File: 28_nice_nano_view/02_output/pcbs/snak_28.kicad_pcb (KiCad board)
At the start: 2 copper layers, 114.8 x 99.6 mm, 156 parts

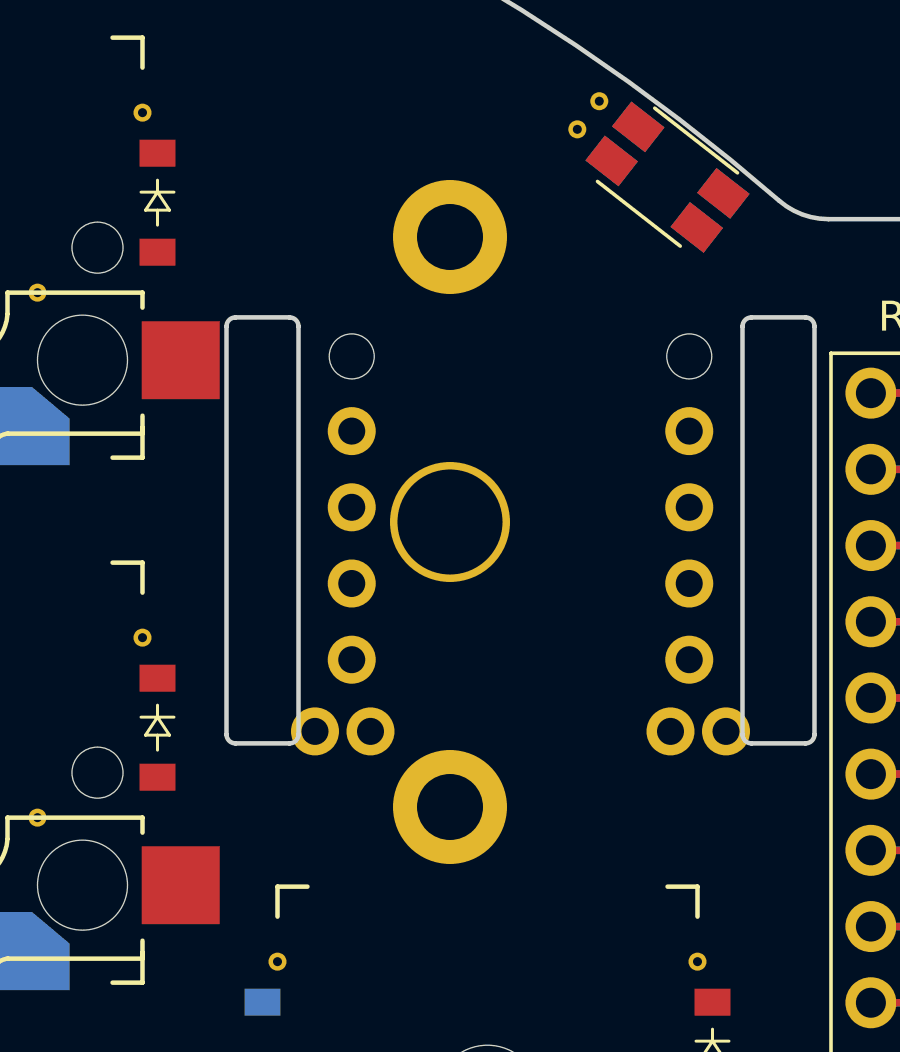
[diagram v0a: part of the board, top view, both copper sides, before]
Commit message: update
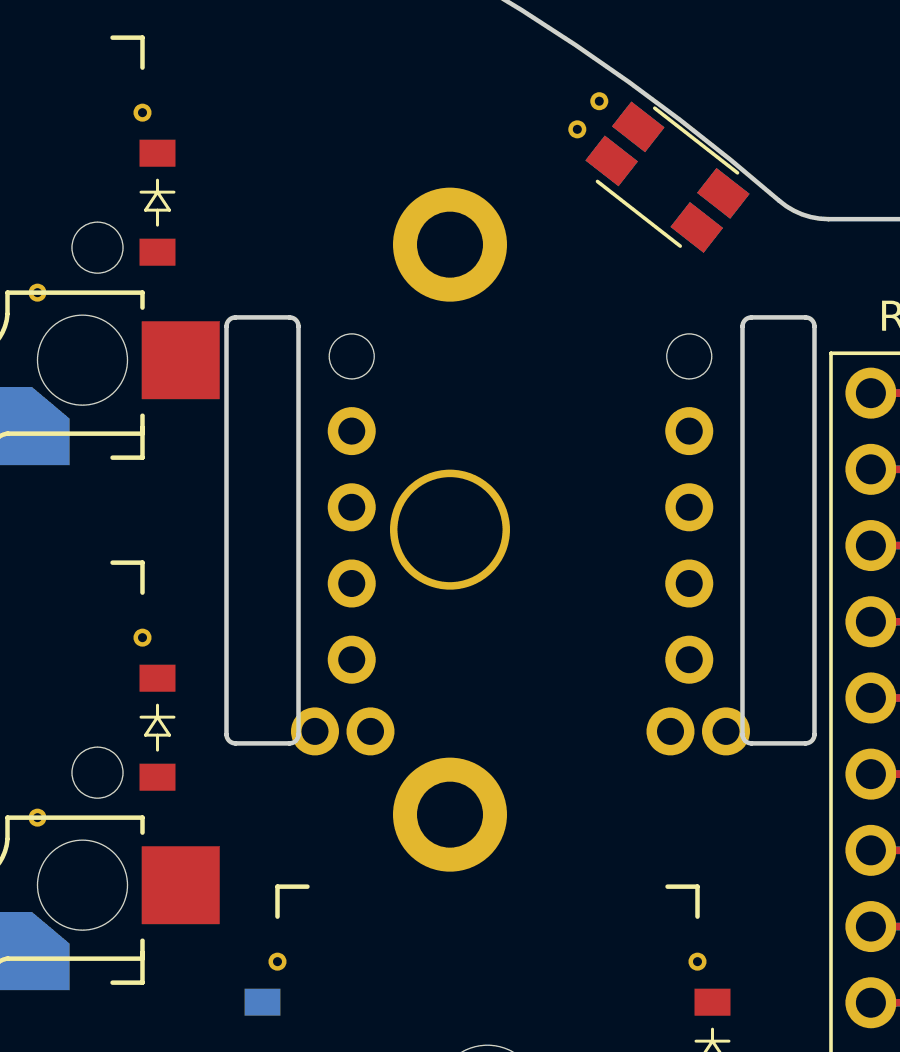
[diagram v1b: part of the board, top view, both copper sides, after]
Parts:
- moved TP1 0.26 mm to (172.8, 62.1)
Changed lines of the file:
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@@
             )
       (module trackpoint_mount_t430 (layer F.Cu)
-        (at 172.75 61.845 0)
+        (at 172.75 62.1 0)
         (attr virtual)
         (fp_text reference "TP1" (at 0 0) (layer B.SilkS) hide
@@
 (gr_circle (center 170.43886559999999 124.35568) (end 171.43886559999999 124.35568) (layer Eco1.User) (width 0.15))
 (gr_circle (center 201.925 53.975) (end 202.925 53.975) (layer Eco1.User) (width 0.15))
-(gr_circle (center 172.75 52.345) (end 173.75 52.345) (layer Eco1.User) (width 0.15))
-(gr_circle (center 172.75 71.345) (end 173.75 71.345) (layer Eco1.User) (width 0.15))
+(gr_circle (center 172.75 52.6) (end 173.75 52.6) (layer Eco1.User) (width 0.15))
+(gr_circle (center 172.75 71.6) (end 173.75 71.6) (layer Eco1.User) (width 0.15))
 (gr_line (start 93.05 89.45) (end 106.95 89.45) (angle 90) (layer Eco1.User) (width 0.15))
 (gr_line (start 106.95 89.45) (end 106.95 75.55) (angle 90) (layer Eco1.User) (width 0.15))
@@
 (gr_circle (center 170.43886559999999 124.35568) (end 171.93886559999999 124.35568) (layer Eco2.User) (width 0.15))
 (gr_circle (center 201.925 53.975) (end 203.425 53.975) (layer Eco2.User) (width 0.15))
-(gr_circle (center 172.75 52.345) (end 174.25 52.345) (layer Eco2.User) (width 0.15))
-(gr_circle (center 172.75 71.345) (end 174.25 71.345) (layer Eco2.User) (width 0.15))
+(gr_circle (center 172.75 52.6) (end 174.25 52.6) (layer Eco2.User) (width 0.15))
+(gr_circle (center 172.75 71.6) (end 174.25 71.6) (layer Eco2.User) (width 0.15))
 )
